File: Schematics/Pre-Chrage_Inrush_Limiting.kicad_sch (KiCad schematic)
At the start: 4 parts, among them Q2 STB10NK60ZT4

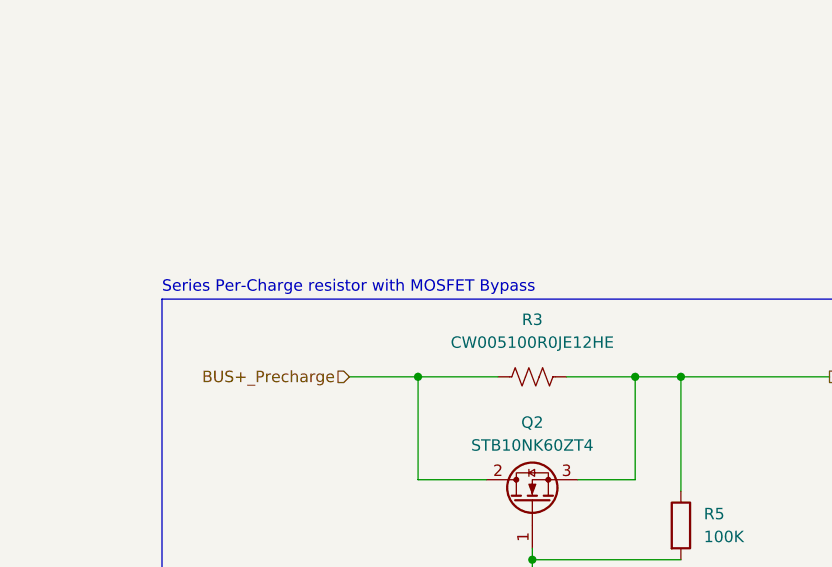
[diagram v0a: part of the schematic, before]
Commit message: Changing Text to Text Block
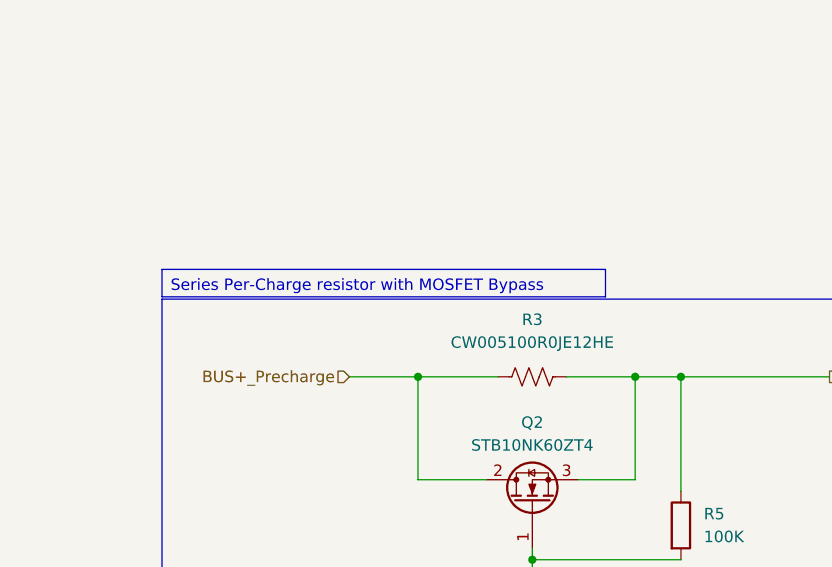
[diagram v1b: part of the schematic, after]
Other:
- note removed: "Series Per-Charge resistor with MOSFET Bypass"
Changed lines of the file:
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@@
-		)
-	)
-	(text "Series Per-Charge resistor with MOSFET Bypass"
-		(exclude_from_sim no)
-		(at 140.462 71.374 0)
-		(effects
-			(font
-				(size 1.27 1.27)
-			)
-			(justify left)
 		)
 	)
@@
 		)
 	)
+	(text_box "Series Per-Charge resistor with MOSFET Bypass"
+		(exclude_from_sim no)
+		(at 140.462 69.342 0)
+		(size 49.276 3.048)
+		(margins 0.9525 0.9525 0.9525 0.9525)
+		(stroke
+			(width 0)
+			(type solid)
+		)
+		(fill
+			(type color)
+			(color 0 0 255 0.1)
+		)
+		(effects
+			(font
+				(size 1.27 1.27)
+			)
+			(justify left top)
+		)
+	)
